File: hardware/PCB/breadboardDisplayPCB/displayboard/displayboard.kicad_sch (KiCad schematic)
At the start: 55 parts, among them J1 Conn_01x09_Socket, Q1 2N7002, Q2 TEPT5700, U1 74HC595, U2 74HC595, U3 74HC595, U4 74HC595, U5 74HC595, U6 TBD62783A, U7 TBD62783A, U8 ULN2803A, U9 ULN2803A

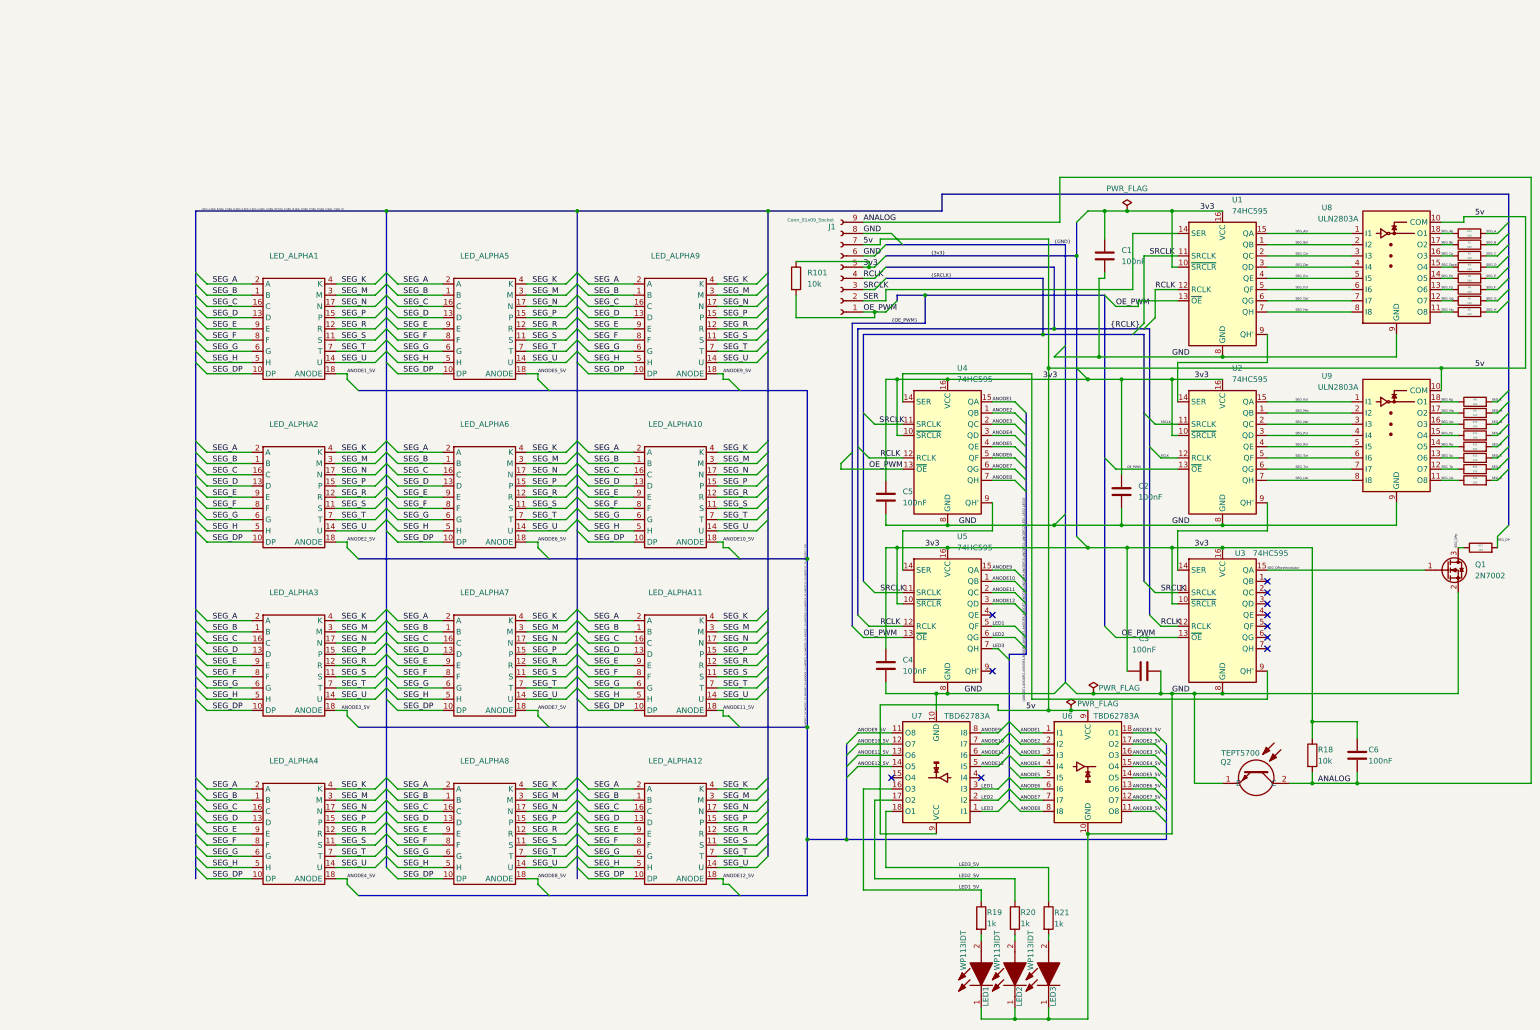
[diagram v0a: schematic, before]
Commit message: large commit of PCB progress
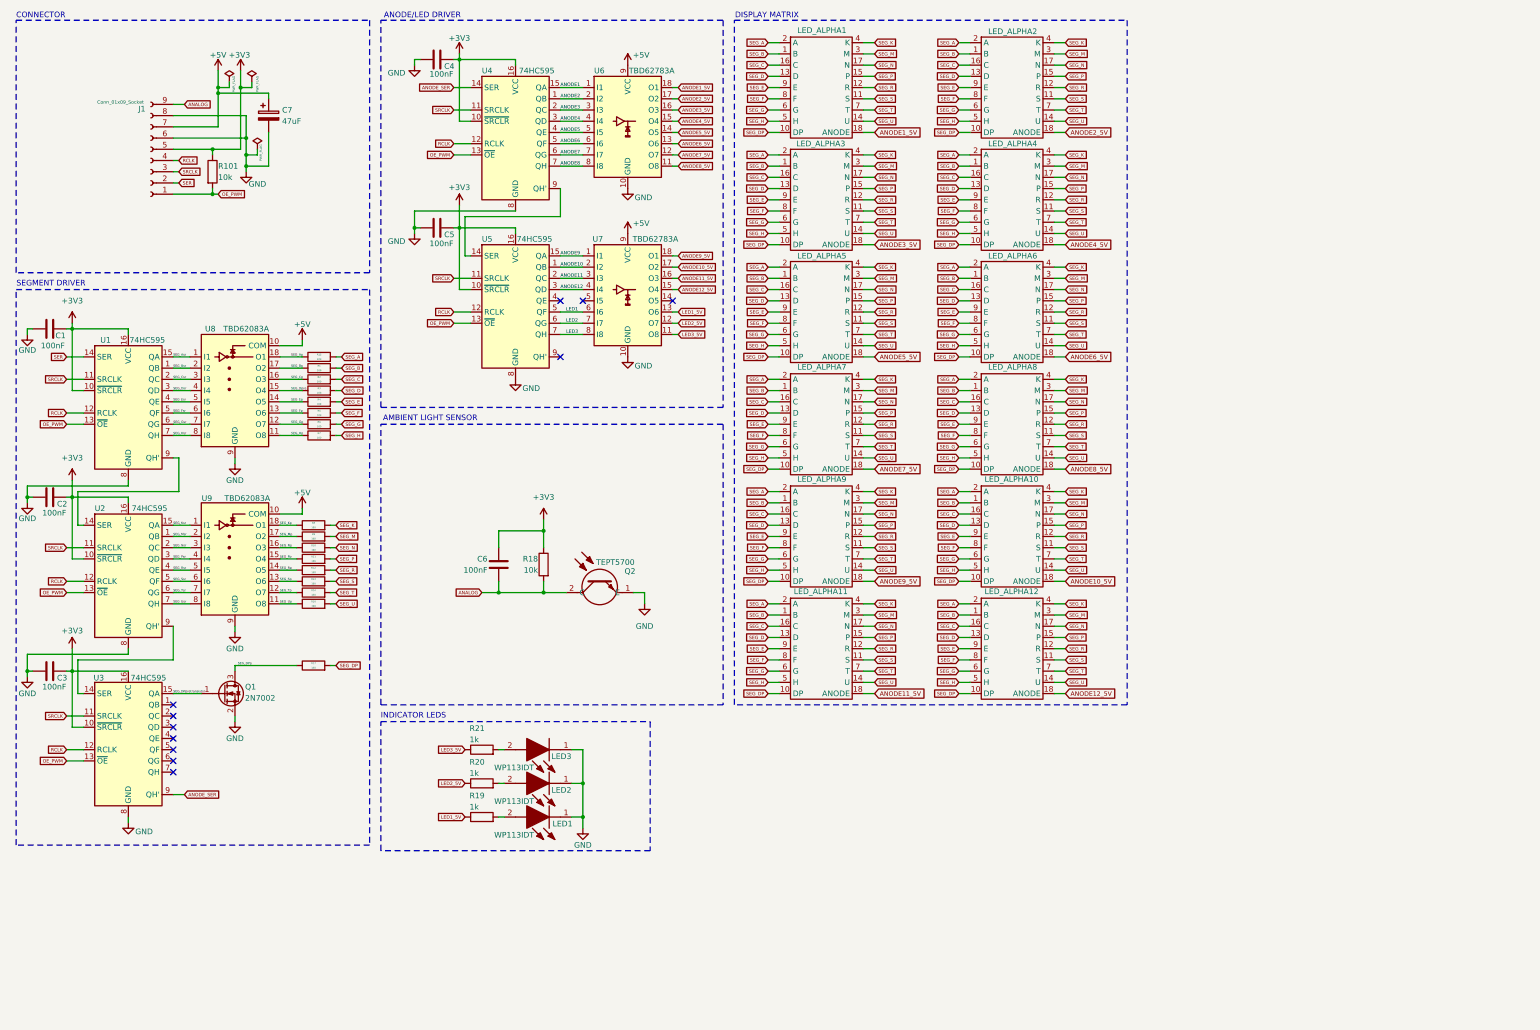
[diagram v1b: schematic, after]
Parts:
- added C7: 47uF, Capacitor_SMD:CP_Elec_6.3x5.4, symbol Device:C_Polarized
- C1, C2, C3, C6: LCSC (none) -> C14663
- C4: renamed from C5; LCSC (none) -> C14663
- C5: renamed from C4; LCSC (none) -> C14663
- J1, LED1, LED2, LED3, LED_ALPHA1, LED_ALPHA12, Q2: now left out of the parts list
- LED_ALPHA10: renamed from LED_ALPHA4; now left out of the parts list
- LED_ALPHA11: renamed from LED_ALPHA8; now left out of the parts list
- LED_ALPHA2: renamed from LED_ALPHA5; now left out of the parts list
- LED_ALPHA3: renamed from LED_ALPHA9; now left out of the parts list
- LED_ALPHA4: renamed from LED_ALPHA2; now left out of the parts list
- LED_ALPHA5: renamed from LED_ALPHA6; now left out of the parts list
- LED_ALPHA6: renamed from LED_ALPHA10; now left out of the parts list
- LED_ALPHA7: renamed from LED_ALPHA3; now left out of the parts list
- LED_ALPHA8: renamed from LED_ALPHA7; now left out of the parts list
- LED_ALPHA9: renamed from LED_ALPHA11; now left out of the parts list
- Q1: LCSC (none) -> C8545
- R1, R10, R11, R12, R13, R14, R15, R16, R17, R2, R3, R4, R5, R6, R7, R8, R9: LCSC (none) -> C17467
- R101: LCSC (none) -> C25804
- R18: LCSC (none) -> C17414
- R19, R20, R21: LCSC (none) -> C21122
- U1, U2, U3, U4, U5: LCSC (none) -> C14791
- U6, U7: LCSC (none) -> C96336
- U8, U9: value ULN2803A -> TBD62083A; LCSC (none) -> C134547
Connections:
- net ANODE10: now also U7.2 (I2); no longer U7.7 (I7)
- net ANODE10_5V: now also LED_ALPHA10.18 (ANODE), U7.17 (O2); no longer LED_ALPHA6.18 (ANODE), U7.12 (O7)
- net ANODE11: now also U7.3 (I3); no longer U7.6 (I6)
- net ANODE11_5V: now also LED_ALPHA11.18 (ANODE), U7.16 (O3); no longer LED_ALPHA9.18 (ANODE), U7.13 (O6)
- net ANODE12: now also U7.4 (I4); no longer U7.5 (I5)
- net ANODE12_5V: now also U7.15 (O4); no longer U7.14 (O5)
- net ANODE2_5V: now also LED_ALPHA2.18 (ANODE); no longer LED_ALPHA4.18 (ANODE)
- net ANODE3_5V: now also LED_ALPHA3.18 (ANODE); no longer LED_ALPHA7.18 (ANODE)
- net ANODE4_5V: now also LED_ALPHA4.18 (ANODE); no longer LED_ALPHA10.18 (ANODE)
- net ANODE5_5V: now also LED_ALPHA5.18 (ANODE); no longer LED_ALPHA2.18 (ANODE)
- net ANODE6_5V: now also LED_ALPHA6.18 (ANODE); no longer LED_ALPHA5.18 (ANODE)
- net ANODE7_5V: now also LED_ALPHA7.18 (ANODE); no longer LED_ALPHA8.18 (ANODE)
- net ANODE8_5V: now also LED_ALPHA8.18 (ANODE); no longer LED_ALPHA11.18 (ANODE)
- net ANODE9: now also U7.1 (I1); no longer U7.8 (I8)
- net ANODE9_5V: now also LED_ALPHA9.18 (ANODE), U7.18 (O1); no longer LED_ALPHA3.18 (ANODE), U7.11 (O8)
- net GND: now also C2.1, C3.1, C4.2, C5.2, C7.2; no longer C2.2, C3.2, C4.1, C5.1
- net LED1: now also U7.6 (I6); no longer U7.3 (I3)
- net LED1_5V: now also U7.13 (O6); no longer U7.16 (O3)
- net LED2: now also U7.7 (I7); no longer U7.2 (I2)
- net LED2_5V: now also U7.12 (O7); no longer U7.17 (O2)
- net LED3: now also U7.8 (I8); no longer U7.1 (I1)
- net LED3_5V: now also U7.11 (O8); no longer U7.18 (O1)
- net ANODE_SER: now reaches U3.9 (QH'), U4.14 (SER)
- net 3v3 renamed +3V3
- net +3V3: now also C2.2, C3.2, C4.1, C5.1; no longer C2.1, C3.1, C4.2, C5.2
- net 5v renamed +5V
- net +5V: now also C7.1
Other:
- note added: "AMBIENT LIGHT SENSOR"
- note added: "ANODE/LED DRIVER"
- note added: "CONNECTOR"
- note added: "DISPLAY MATRIX"
- note added: "INDICATOR LEDS"
- note added: "SEGMENT DRIVER"
- company: (none) -> NATHANIEL KESSEL
- moved on the sheet: C1, C2, C3, C4, C5, C6, J1, LED1, LED2, LED3, LED_ALPHA1, LED_ALPHA10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
